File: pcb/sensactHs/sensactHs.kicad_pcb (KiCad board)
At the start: 2 copper layers, 100 x 86.5 mm, 185 parts, among them M1 Hole, M2 Hole, P1 CONN_01X08, P2 USB, P3 ESP01, P4 MicroSD, P5 SWD, P6 PWR+CANH, P7 CANH+CANL, P8 !24V!, SW1 PC5-Key, SW2 BOOT0, SW3 RESET, SW4 BOOT1, U1 ULN2803, U10 SRV05, U11 SRV05, U12 SRV05, U13 SRV05, U14 SRV05, U15 SRV05, U16 SRV05, U17 SRV05, U18 PCA9555, U19 PCA9555, U2 DRV8860woPad, U20 DRV8860woPad, U3 DRV8860woPad, U4 STM32F103RG, U5 LM2674, U6 SN65HVD230, U7 PCA9685, U8 DS2482, U9 PCA9685, X1 8MHz

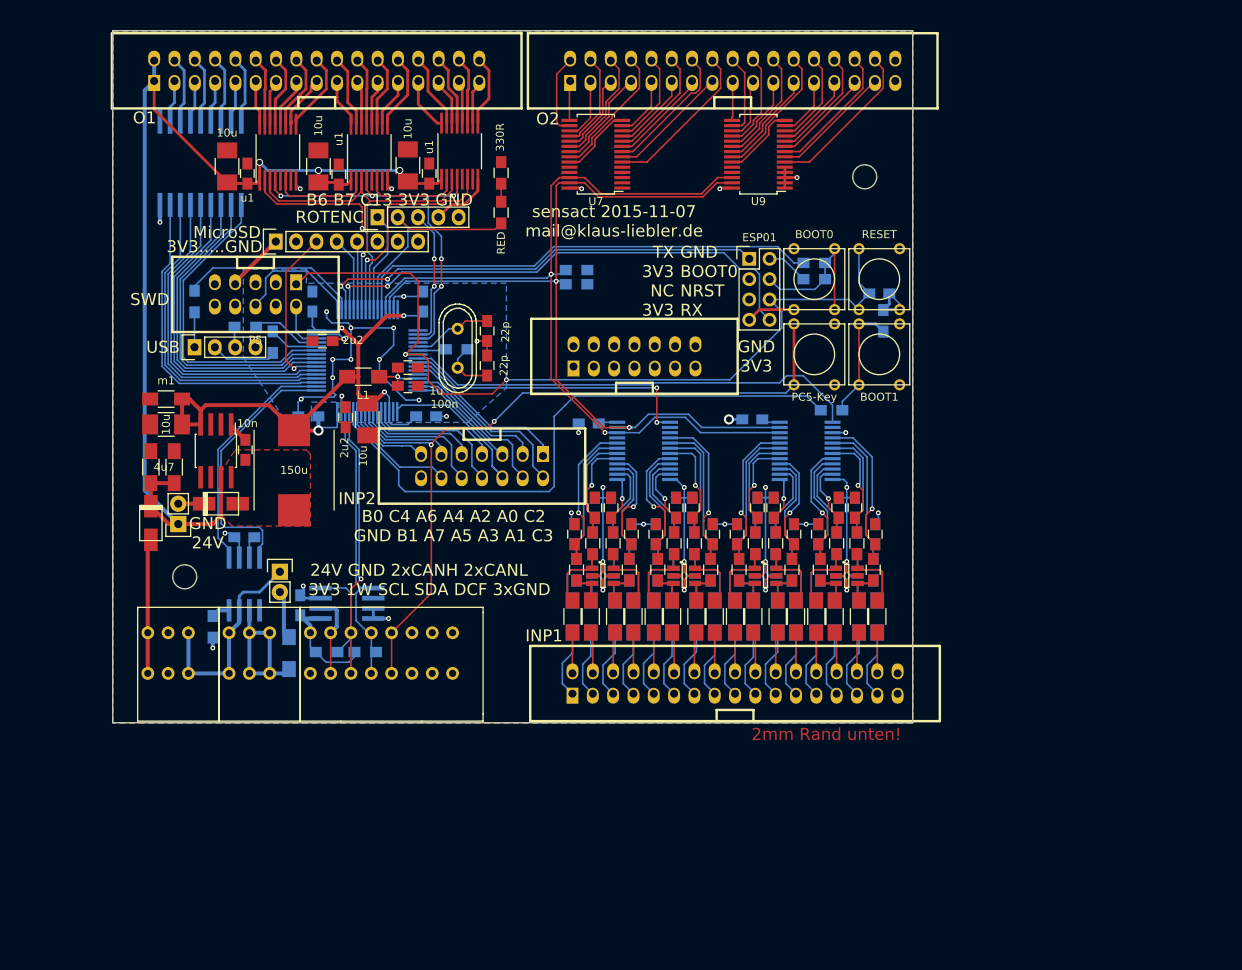
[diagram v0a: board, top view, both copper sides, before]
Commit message: new version of sensactHs
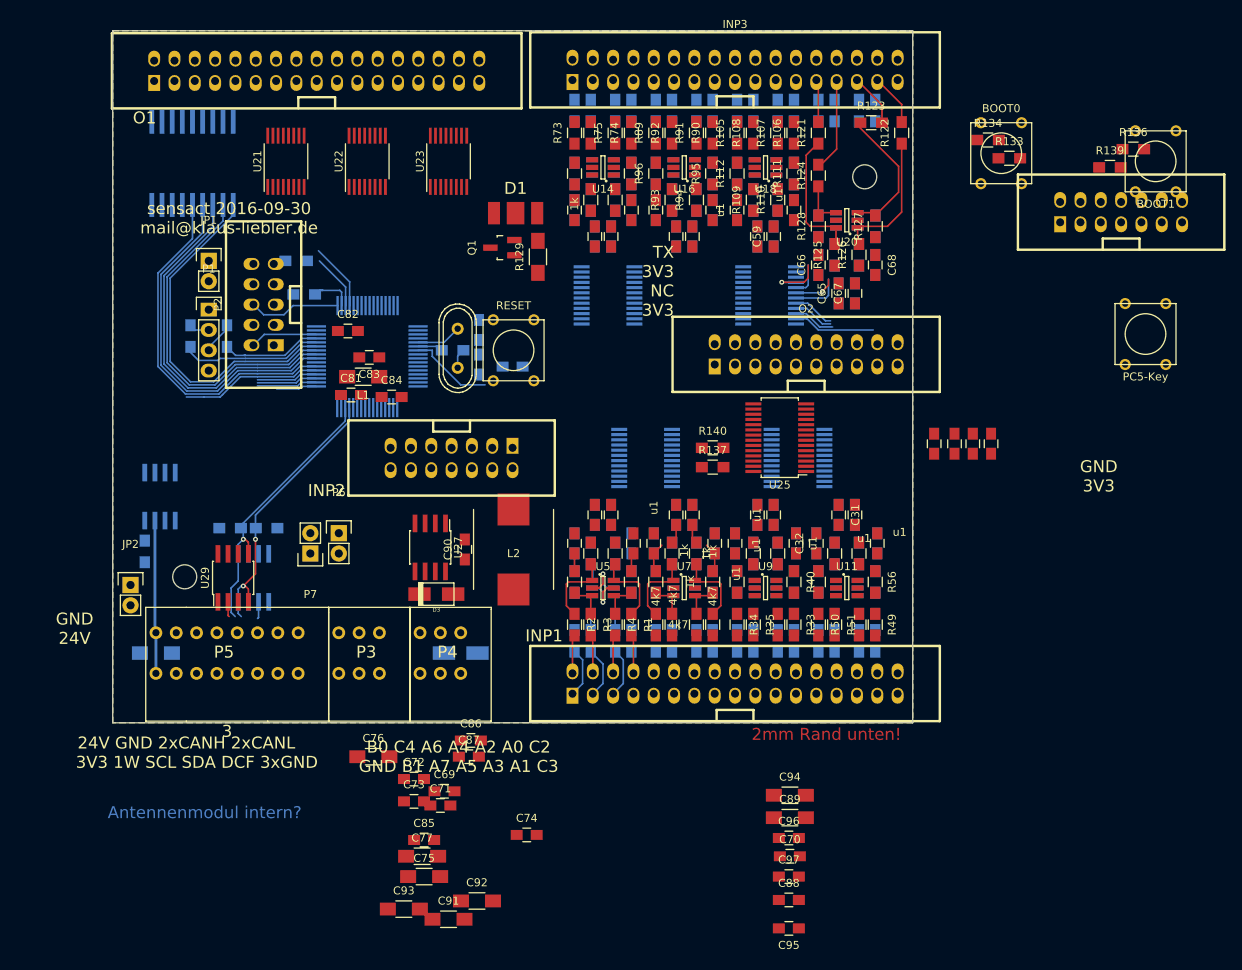
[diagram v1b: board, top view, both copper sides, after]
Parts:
- removed D16: RED, Resistors_SMD:R_0805_HandSoldering
- removed D17: SS14, kl_footprints:do214ac_handsolder
- removed D18: MBR0540, kl_footprints:do214ac_handsolder
- removed INP4: ROTENC, Pin_Headers:Pin_Header_Straight_1x05
- removed JP3: CAN_TERM, Pin_Headers:Pin_Header_Straight_1x02
- removed P8: !24V!, Pin_Headers:Pin_Header_Straight_1x02
- added C60: u1, Capacitors_SMD:C_0805_HandSoldering, F.Cu at (105.2, 41.9)
- added C61: u1, Capacitors_SMD:C_0805_HandSoldering, B.Cu at (112.8, 52.3)
- added C62: u1, Capacitors_SMD:C_0805_HandSoldering, B.Cu at (115.3, 48.8)
- added C63: u1, Capacitors_SMD:C_0805_HandSoldering, B.Cu at (110.7, 52.3)
- added C64: u1, Capacitors_SMD:C_0805_HandSoldering, B.Cu at (108.2, 48.8)
- added C65: u1, Capacitors_SMD:C_0805_HandSoldering, F.Cu at (110.7, 52.3)
- added C66: u1, Capacitors_SMD:C_0805_HandSoldering, F.Cu at (108.2, 48.8)
- added C67: u1, Capacitors_SMD:C_0805_HandSoldering, F.Cu at (112.8, 52.3)
- added C68: u1, Capacitors_SMD:C_0805_HandSoldering, F.Cu at (115.3, 48.8)
- added C69: u1, Capacitors_SMD:C_0805_HandSoldering, F.Cu at (61.5, 114.6)
- added C70: u1, Capacitors_SMD:C_0805_HandSoldering, F.Cu at (104.6, 122.7)
- added C71: u1, Capacitors_SMD:C_0805_HandSoldering, F.Cu at (61.0, 116.3)
- added C72: u1, Capacitors_SMD:C_0805_HandSoldering, F.Cu at (57.7, 113.0)
- added C73: u1, Capacitors_SMD:C_0805_HandSoldering, F.Cu at (57.7, 115.8)
- added C74: u1, Capacitors_SMD:C_0805_HandSoldering, F.Cu at (71.8, 120.0)
- added C75: 10u, Capacitors_SMD:C_1206_HandSoldering, F.Cu at (58.9, 125.2)
- added C76: 10u, Capacitors_SMD:C_1206_HandSoldering, F.Cu at (52.6, 110.2)
- added C77: 10u, Capacitors_SMD:C_1206_HandSoldering, F.Cu at (58.7, 122.7)
- added C78: 22p, Capacitors_SMD:C_0805_HandSoldering, B.Cu at (65.8, 56.9)
- added C79: 22p, Capacitors_SMD:C_0805_HandSoldering, B.Cu at (65.8, 61.2)
- added C80: u1, Capacitors_SMD:C_0805_HandSoldering, B.Cu at (70.0, 61.5)
- added C81: 2u2, Capacitors_SMD:C_0805_HandSoldering, F.Cu at (49.8, 65.0)
- added C82: 2u2, Capacitors_SMD:C_0805_HandSoldering, F.Cu at (49.4, 57.0)
- added C83: 1u, Capacitors_SMD:C_0805_HandSoldering, F.Cu at (52.1, 60.3)
- added C84: 1u, Capacitors_SMD:C_0805_HandSoldering, F.Cu at (54.9, 65.3)
- added C85: u1, Capacitors_SMD:C_0805_HandSoldering, F.Cu at (58.9, 120.7)
- added C86: u1, Capacitors_SMD:C_0805_HandSoldering, F.Cu at (64.8, 108.2)
- added C87: u1, Capacitors_SMD:C_0805_HandSoldering, F.Cu at (64.5, 110.2)
- added C88: u1, Capacitors_SMD:C_0805_HandSoldering, F.Cu at (104.5, 128.1)
- added C89: 10u, Capacitors_SMD:C_1206_HandSoldering, F.Cu at (104.6, 117.9)
- added C90: 10n, Capacitors_SMD:C_0805_HandSoldering, F.Cu at (64.0, 84.3)
- added C91: 4u7, Capacitors_SMD:C_1206_HandSoldering, F.Cu at (62.0, 130.6)
- added C92: 4u7, Capacitors_SMD:C_1206_HandSoldering, F.Cu at (65.5, 128.3)
- added C93: 10u, Capacitors_SMD:C_1206_HandSoldering, F.Cu at (56.4, 129.3)
- added C94: m1, Capacitors_SMD:C_1206_HandSoldering, F.Cu at (104.6, 115.1)
- added C95: 100n, Capacitors_SMD:C_0805_HandSoldering, F.Cu at (104.5, 131.7)
- added C96: u1, Capacitors_SMD:C_0805_HandSoldering, F.Cu at (104.5, 120.4)
- added C97: u1, Capacitors_SMD:C_0805_HandSoldering, F.Cu at (104.5, 125.2)
- added D1: RED, sensact:LED_5730, F.Cu at (70.4, 42.3)
- added D2: D, sensact:do214ac_handsolder, B.Cu at (63.5, 97.3)
- added D3: MBR0540, sensact:do214ac_handsolder, F.Cu at (60.5, 89.9)
- added INP3: PUSH_BUTTON_INPUT, w_conn_strip:vasch_strip_17x2, F.Cu at (97.8, 24.4)
- added JP1: JUMPER, Pin_Headers:Pin_Header_Straight_1x02, F.Cu at (32.0, 48.3)
- added JP2: CAN_TERM, Pin_Headers:Pin_Header_Straight_1x02, F.Cu at (22.2, 88.8)
- added Q1: Q_NPN_BEC, TO_SOT_Packages_SMD:SOT-23_Handsoldering, F.Cu at (68.7, 46.6)
- added R100: 4k7, Resistors_SMD:R_0805_HandSoldering, B.Cu at (103.1, 29.5)
- added R101: 1k, Resistors_SMD:R_0805_HandSoldering, B.Cu at (103.1, 40.6)
- added R102: 1k, Resistors_SMD:R_0805_HandSoldering, B.Cu at (100.1, 40.6)
- added R103: 1k, Resistors_SMD:R_0805_HandSoldering, B.Cu at (98.0, 37.3)
- added R104: 1k, Resistors_SMD:R_0805_HandSoldering, B.Cu at (105.2, 37.3)
- added R105: 4k7, Resistors_SMD:R_0805_HandSoldering, F.Cu at (98.0, 32.3)
- added R106: 4k7, Resistors_SMD:R_0805_HandSoldering, F.Cu at (105.2, 32.3)
- added R107: 4k7, Resistors_SMD:R_0805_HandSoldering, F.Cu at (103.1, 32.3)
- added R108: 4k7, Resistors_SMD:R_0805_HandSoldering, F.Cu at (100.1, 32.3)
- added R109: 1k, Resistors_SMD:R_0805_HandSoldering, F.Cu at (100.1, 40.6)
- added R110: 1k, Resistors_SMD:R_0805_HandSoldering, F.Cu at (103.1, 40.6)
- added R111: 1k, Resistors_SMD:R_0805_HandSoldering, F.Cu at (105.2, 37.3)
- added R112: 1k, Resistors_SMD:R_0805_HandSoldering, F.Cu at (98.0, 37.3)
- added R113: 4k7, Resistors_SMD:R_0805_HandSoldering, B.Cu at (115.3, 29.5)
- added R114: 4k7, Resistors_SMD:R_0805_HandSoldering, B.Cu at (108.2, 29.5)
- added R115: 4k7, Resistors_SMD:R_0805_HandSoldering, B.Cu at (110.2, 29.5)
- added R116: 4k7, Resistors_SMD:R_0805_HandSoldering, B.Cu at (113.3, 29.5)
- added R117: 1k, Resistors_SMD:R_0805_HandSoldering, B.Cu at (113.3, 47.5)
- added R118: 1k, Resistors_SMD:R_0805_HandSoldering, B.Cu at (110.2, 47.5)
- added R119: 1k, Resistors_SMD:R_0805_HandSoldering, B.Cu at (108.2, 43.9)
- added R120: 1k, Resistors_SMD:R_0805_HandSoldering, B.Cu at (115.3, 43.9)
- added R121: 4k7, Resistors_SMD:R_0805_HandSoldering, F.Cu at (108.2, 32.3)
- added R122: 4k7, Resistors_SMD:R_0805_HandSoldering, F.Cu at (118.6, 32.3)
- added R123: 4k7, Resistors_SMD:R_0805_HandSoldering, F.Cu at (114.8, 31.0)
- added R124: 4k7, Resistors_SMD:R_0805_HandSoldering, F.Cu at (108.2, 37.6)
- added R125: 1k, Resistors_SMD:R_0805_HandSoldering, F.Cu at (110.2, 47.5)
- added R126: 1k, Resistors_SMD:R_0805_HandSoldering, F.Cu at (113.3, 47.5)
- added R127: 1k, Resistors_SMD:R_0805_HandSoldering, F.Cu at (115.3, 43.9)
- added R128: 1k, Resistors_SMD:R_0805_HandSoldering, F.Cu at (108.2, 43.9)
- added R129: 330R, Resistors_SMD:R_1206_HandSoldering, F.Cu at (73.2, 47.8)
- added R130: 1k, Resistors_SMD:R_0805_HandSoldering, B.Cu at (43.9, 52.5)
- added R131: 22R, Resistors_SMD:R_0805_HandSoldering, B.Cu at (29.7, 57.7)
- added R132: 22R, Resistors_SMD:R_0805_HandSoldering, B.Cu at (34.3, 57.7)
- added R133: 10k, Resistors_SMD:R_0805_HandSoldering, F.Cu at (132.1, 35.4)
- added R134: 10k, Resistors_SMD:R_0805_HandSoldering, F.Cu at (129.4, 33.1)
- added R135: 220R, Resistors_SMD:R_0805_HandSoldering, B.Cu at (62.5, 59.4)
- added R136: 10k, Resistors_SMD:R_0805_HandSoldering, F.Cu at (147.6, 34.3)
- added R137: 4k7, Resistors_SMD:R_0805_HandSoldering, F.Cu at (95.0, 74.0)
- added R138: 4k7, Resistors_SMD:R_0805_HandSoldering, B.Cu at (39.2, 81.7)
- added R139: 10k, Resistors_SMD:R_0805_HandSoldering, F.Cu at (144.7, 36.6)
- added R140: 4k7, Resistors_SMD:R_0805_HandSoldering, F.Cu at (95.0, 71.6)
- added R141: 4k7, Resistors_SMD:R_0805_HandSoldering, B.Cu at (34.7, 81.7)
- added R142: 10k, Resistors_SMD:R_0805_HandSoldering, B.Cu at (24.0, 84.6)
- added R143: 120R, Resistors_SMD:R_1206_HandSoldering, B.Cu at (25.4, 97.3)
- added R144: 1k, Resistors_SMD:R_0805_HandSoldering, B.Cu at (42.9, 48.3)
- added R28: 4k7, Resistors_SMD:R_0805_HandSoldering, B.Cu at (89.9, 95.8)
- added R29: 1k, Resistors_SMD:R_0805_HandSoldering, B.Cu at (89.9, 84.8)
- added R82: 4k7, Resistors_SMD:R_0805_HandSoldering, B.Cu at (87.9, 29.5)
- added R83: 4k7, Resistors_SMD:R_0805_HandSoldering, B.Cu at (89.9, 29.5)
- added R84: 4k7, Resistors_SMD:R_0805_HandSoldering, B.Cu at (93.0, 29.5)
- added R85: 1k, Resistors_SMD:R_0805_HandSoldering, B.Cu at (93.0, 40.6)
- added R86: 1k, Resistors_SMD:R_0805_HandSoldering, B.Cu at (89.9, 40.6)
- added R87: 1k, Resistors_SMD:R_0805_HandSoldering, B.Cu at (87.9, 37.3)
- added R88: 1k, Resistors_SMD:R_0805_HandSoldering, B.Cu at (95.0, 37.3)
- added R89: 4k7, Resistors_SMD:R_0805_HandSoldering, F.Cu at (87.9, 32.3)
- added R90: 4k7, Resistors_SMD:R_0805_HandSoldering, F.Cu at (95.0, 32.3)
- added R91: 4k7, Resistors_SMD:R_0805_HandSoldering, F.Cu at (93.0, 32.3)
- added R92: 4k7, Resistors_SMD:R_0805_HandSoldering, F.Cu at (89.9, 32.3)
- added R93: 1k, Resistors_SMD:R_0805_HandSoldering, F.Cu at (89.9, 40.6)
- added R94: 1k, Resistors_SMD:R_0805_HandSoldering, F.Cu at (93.0, 40.6)
- added R95: 1k, Resistors_SMD:R_0805_HandSoldering, F.Cu at (95.0, 37.3)
- added R96: 1k, Resistors_SMD:R_0805_HandSoldering, F.Cu at (87.9, 37.3)
- added R97: 4k7, Resistors_SMD:R_0805_HandSoldering, B.Cu at (105.2, 29.5)
- added R98: 4k7, Resistors_SMD:R_0805_HandSoldering, B.Cu at (98.0, 29.5)
- added R99: 4k7, Resistors_SMD:R_0805_HandSoldering, B.Cu at (100.1, 29.5)
- added U21: DRV8860woPad, sensact:TSSOP-16_4.4x5mm_Pitch0.65mm_handsolder, F.Cu at (41.7, 35.8)
- added U22: DRV8860woPad, sensact:TSSOP-16_4.4x5mm_Pitch0.65mm_handsolder, F.Cu at (51.8, 35.8)
- added U23: DRV8860woPad, sensact:TSSOP-16_4.4x5mm_Pitch0.65mm_handsolder, F.Cu at (62.0, 35.8)
- added U24: ULN2803, sensact:SOIC-18_7.5x11.6mm_Pitch1.27mm_handsolder, B.Cu at (30.0, 36.1)
- added U25: PCA9685, sensact:TSSOP-28_4.4x9.7mm_Pitch0.65mm_handsolder, F.Cu at (103.4, 70.4)
- added U26: STM32F103RG, sensact:LQFP-64_10x10mm_Pitch0.5mm_handsolder, B.Cu at (51.8, 60.2)
- added U27: LM2674, sensact:SOIC-8_3.9x4.9mm_Pitch1.27mm_handsolder, F.Cu at (59.7, 84.1)
- added U28: SN65HVD230, sensact:SOIC-8_3.9x4.9mm_Pitch1.27mm_handsolder, B.Cu at (25.9, 77.7)
- added U29: DS2482, sensact:SOIC-8_3.9x4.9mm_Pitch1.27mm_handsolder, F.Cu at (35.1, 87.9)
- added U30: DS2482, sensact:SOIC-8_3.9x4.9mm_Pitch1.27mm_handsolder, B.Cu at (37.6, 87.9)
- C10, C11, C12, C17, C40, C45, C53, C9, R69, R70, R71: moved to B.Cu
- C13, C14, C15, C41, C49, C5, C57, C58, C6, C7, C8, R77, R78, R79: moved to F.Cu
- C18, C19, C36: value 10u -> u1; footprint Capacitors_SMD:C_1210_HandSoldering -> Capacitors_SMD:C_0805_HandSoldering; moved to B.Cu
- C20: value 22p -> u1; moved to B.Cu
- C21: value 22p -> u1
- C22, C29, C30: value 100n -> u1; moved to F.Cu
- C23, C24: value 2u2 -> u1
- C25: value 100n -> u1; moved to B.Cu
- C26: value 1u -> u1; moved to B.Cu
- C27, C28, C38: value 100n -> u1
- C31, C59: value 10u -> u1; footprint Capacitors_SMD:C_1210_HandSoldering -> Capacitors_SMD:C_0805_HandSoldering
- C32: value 4u7 -> u1; footprint Capacitors_SMD:C_1206_HandSoldering -> Capacitors_SMD:C_0805_HandSoldering
- C33: value 4u7 -> u1; footprint Capacitors_SMD:C_1206_HandSoldering -> Capacitors_SMD:C_0805_HandSoldering; moved to B.Cu
- C34: value 10n -> u1; moved to B.Cu
- C37: value m1 -> u1; footprint Capacitors_SMD:C_1206_HandSoldering -> Capacitors_SMD:C_0805_HandSoldering; moved to B.Cu
- L2: footprint kl_footprints:Inductor_CD104_handsolder -> sensact:Inductor_CD104_handsolder
- O2: value PWM OUTPUTS -> PWM_OUTPUTS; footprint w_conn_strip:vasch_strip_17x2 -> w_conn_strip:vasch_strip_10x2
- P1: value CONN_01X08 -> USB; footprint kl_footprints:KF141R-8p -> Pin_Headers:Pin_Header_Straight_1x04
- P2: value USB -> SWD; footprint Pin_Headers:Pin_Header_Straight_1x04 -> w_conn_strip:vasch_strip_5x2
- P3: value ESP01 -> 2; footprint Pin_Headers:Pin_Header_Straight_2x04 -> sensact:KF141R-3p
- P4: value MicroSD -> 1; footprint Pin_Headers:Pin_Header_Straight_1x08 -> sensact:KF141R-3p
- P5: value SWD -> 3; footprint w_conn_strip:vasch_strip_5x2 -> sensact:KF141R-8p
- P6: value PWR+CANH -> !24V!; footprint kl_footprints:KF141R-3p -> Pin_Headers:Pin_Header_Straight_1x02
- P7: value CANH+CANL -> 5V_IN; footprint kl_footprints:KF141R-3p -> Pin_Headers:Pin_Header_Straight_1x02
- R1, R10, R11, R12, R2, R3, R33, R34, R35, R4, R41, R42, R43, R49, R50, R51, R57, R58, R59, R9: footprint Resistors_SMD:R_1206_HandSoldering -> Resistors_SMD:R_0805_HandSoldering
- R16: value 330R -> 1k; moved to B.Cu
- R17, R18: value 22R -> 4k7; moved to F.Cu
- R19, R20: value 10k -> 4k7; moved to F.Cu
- R21: value 220R -> 1k; moved to F.Cu
- R22, R23, R80: value 4k7 -> 1k; moved to F.Cu
- R24: value 10k -> 1k; moved to F.Cu
- R25, R26: value 10k -> 4k7
- R27: value 120R -> 4k7; footprint Resistors_SMD:R_1206_HandSoldering -> Resistors_SMD:R_0805_HandSoldering
- R32, R48, R64: value 4k7 -> 1k; footprint Resistors_SMD:R_1206_HandSoldering -> Resistors_SMD:R_0805_HandSoldering; moved to B.Cu
- R36, R44, R52, R60: value 1k -> 4k7
- R40, R56: value 4k7 -> 1k; footprint Resistors_SMD:R_1206_HandSoldering -> Resistors_SMD:R_0805_HandSoldering; moved to F.Cu
- R65, R66, R67: footprint Resistors_SMD:R_1206_HandSoldering -> Resistors_SMD:R_0805_HandSoldering; moved to B.Cu
- R68: value 1k -> 4k7; moved to B.Cu
- R72: value 4k7 -> 1k; footprint Resistors_SMD:R_1206_HandSoldering -> Resistors_SMD:R_0805_HandSoldering
- R73, R74, R75: footprint Resistors_SMD:R_1206_HandSoldering -> Resistors_SMD:R_0805_HandSoldering; moved to F.Cu
- R76: value 1k -> 4k7; moved to F.Cu
- U1: value ULN2803 -> PCA9555; footprint kl_footprints:SOIC-18_7.5x11.6mm_Pitch1.27mm_handsolder -> sensact:TSSOP-24_4.4x7.8mm_Pitch0.65mm_handsolder
- U10, U12: footprint kl_footprints:SOT-23-6_handsolder -> sensact:SOT-23-6_handsolder; moved to B.Cu
- U11: footprint kl_footprints:SOT-23-6_handsolder -> sensact:SOT-23-6_handsolder; moved to F.Cu
- U13, U14, U15, U16, U17: footprint kl_footprints:SOT-23-6_handsolder -> sensact:SOT-23-6_handsolder
- U18: value PCA9555 -> SRV05; footprint kl_footprints:TSSOP-24_4.4x7.8mm_Pitch0.65mm_handsolder -> sensact:SOT-23-6_handsolder; moved to F.Cu
- U19: value PCA9555 -> SRV05; footprint kl_footprints:TSSOP-24_4.4x7.8mm_Pitch0.65mm_handsolder -> sensact:SOT-23-6_handsolder
- U2, U3: value DRV8860woPad -> PCA9555; footprint kl_footprints:TSSOP-16_4.4x5mm_Pitch0.65mm_handsolder -> sensact:TSSOP-24_4.4x7.8mm_Pitch0.65mm_handsolder; moved to B.Cu
- U20: value DRV8860woPad -> SRV05; footprint kl_footprints:TSSOP-16_4.4x5mm_Pitch0.65mm_handsolder -> sensact:SOT-23-6_handsolder
- U4: value STM32F103RG -> PCA9555; footprint kl_footprints:LQFP-64_10x10mm_Pitch0.5mm_handsolder -> sensact:TSSOP-24_4.4x7.8mm_Pitch0.65mm_handsolder
- U5: value LM2674 -> SRV05; footprint kl_footprints:SOIC-8_3.9x4.9mm_Pitch1.27mm_handsolder -> sensact:SOT-23-6_handsolder
- U6: value SN65HVD230 -> SRV05; footprint kl_footprints:SOIC-8_3.9x4.9mm_Pitch1.27mm_handsolder -> sensact:SOT-23-6_handsolder
- U7, U9: value PCA9685 -> SRV05; footprint kl_footprints:TSSOP-28_4.4x9.7mm_Pitch0.65mm_handsolder -> sensact:SOT-23-6_handsolder
- U8: value DS2482 -> SRV05; footprint kl_footprints:SOIC-8_3.9x4.9mm_Pitch1.27mm_handsolder -> sensact:SOT-23-6_handsolder
- moved C36 90.1 mm to (115.6, 83.6), turned to 90 degrees
- moved C32 83.7 mm to (108.0, 83.6)
- moved C33 83.3 mm to (110.7, 80.0), turned to 270 degrees
- moved U2 75.4 mm to (105.7, 72.9), turned to 180 degrees
- moved C29 72.9 mm to (112.8, 80.0), turned to 270 degrees
- moved C19 72.7 mm to (92.5, 80.0), turned to 270 degrees
- moved C34 72.3 mm to (108.0, 83.6)
- moved R67 71.6 mm to (79.8, 29.5), turned to 90 degrees
- moved R73 71.3 mm to (77.7, 32.3), turned to 90 degrees
- moved R66 71.1 mm to (77.7, 29.5), turned to 90 degrees
- moved C35 70.3 mm to (112.8, 80.0), turned to 270 degrees
- moved R30 70.2 mm to (93.0, 84.8), turned to 270 degrees
- moved C17 68.5 mm to (90.4, 80.0), turned to 270 degrees
- moved P3 68.4 mm to (52.1, 97.3)
- moved R65 67.3 mm to (84.8, 29.5), turned to 90 degrees
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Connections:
- C1 pad 1: GND -> +3V3
- C1 pad 2: /01 input/ESDProtection1/O1 -> GND
- C10 pad 1: /01 input/ESDProtection3/O4 -> /01 input/ESDProtection2/O4
- C11 pad 2: /01 input/ESDProtection3/O2 -> /01 input/ESDProtection2/O2
- C12 pad 1: /01 input/ESDProtection3/O3 -> /01 input/ESDProtection2/O3
- C13 pad 2: /01 input/ESDProtection4/O1 -> /01 input/ESDProtection3/O1
- C14 pad 1: /01 input/ESDProtection4/O4 -> /01 input/ESDProtection3/O4
- C15 pad 2: /01 input/ESDProtection4/O2 -> /01 input/ESDProtection3/O2
- C16 pad 1: VCC -> /01 input/ESDProtection3/O3
- C17 pad 1: VCC -> GND
- C17 pad 2: GND -> /01 input/ESDProtection4/O1
- C18 pad 1: VCC -> /01 input/ESDProtection4/O4
- C19 pad 1: VCC -> GND
- C19 pad 2: GND -> /01 input/ESDProtection4/O2
- C2 pad 1: /01 input/ESDProtection1/O4 -> +3V3
- C20 pad 1: Net-(C20-Pad1) -> /01 input/ESDProtection4/O3
- C21 pad 1: Net-(C21-Pad1) -> GND
- C21 pad 2: GND -> /01 input/ESDProtection5/O1
- C22 pad 1: /03 cpu/NRST -> /01 input/ESDProtection5/O4
- C23 pad 1: Net-(C23-Pad1) -> GND
- C23 pad 2: GND -> /01 input/ESDProtection5/O2
- C24 pad 1: Net-(C24-Pad1) -> /01 input/ESDProtection5/O3
- C25 pad 1: Net-(C25-Pad1) -> GND
- C25 pad 2: GND -> /01 input/ESDProtection6/O1
- C26 pad 1: Net-(C25-Pad1) -> /01 input/ESDProtection6/O4
- C27 pad 1: +3V3 -> GND
- C27 pad 2: GND -> /01 input/ESDProtection6/O2
- C28 pad 1: +3V3 -> /01 input/ESDProtection6/O3
- C29 pad 1: +3V3 -> GND
- C29 pad 2: GND -> /01 input/ESDProtection7/O1
- C3 pad 1: GND -> +3V3
- C3 pad 2: /01 input/ESDProtection1/O2 -> GND
- C30 pad 1: +3V3 -> /01 input/ESDProtection7/O4
- C31 pad 1: +3V3 -> GND
- C31 pad 2: GND -> /01 input/ESDProtection7/O2
- C32 pad 1: VCC -> /01 input/ESDProtection7/O3
- C33 pad 1: VCC -> GND
- C33 pad 2: GND -> /01 input/ESDProtection8/O1
- C34 pad 1: /04 power/V_SW -> /01 input/ESDProtection8/O4
- C34 pad 2: /04 power/V_CB -> GND
- C35 pad 1: +3V3 -> GND
- C35 pad 2: GND -> /01 input/ESDProtection8/O2
- C36 pad 1: +3V3 -> /01 input/ESDProtection8/O3
- C37 pad 1: +3V3 -> GND
- C37 pad 2: GND -> /01 input/ESDProtection9/O1
- C38 pad 1: +3V3 -> /01 input/ESDProtection9/O4
- C39 pad 1: +3V3 -> GND
- C39 pad 2: GND -> /01 input/ESDProtection9/O2
- C4 pad 1: /01 input/ESDProtection1/O3 -> +3V3
- C40 pad 1: VCC -> /01 input/ESDProtection9/O3
- C41 pad 1: /01 input/ESDProtection4/O3 -> GND
- C41 pad 2: GND -> /01 input/ESDProtection10/O1
- C42 pad 1: GND -> /01 input/ESDProtection10/O4
- C42 pad 2: /01 input/ESDProtection5/O1 -> GND
- C43 pad 1: /01 input/ESDProtection5/O4 -> GND
- C43 pad 2: GND -> /01 input/ESDProtection10/O2
- C44 pad 1: GND -> /01 input/ESDProtection10/O3
- C44 pad 2: /01 input/ESDProtection5/O2 -> GND
- C45 pad 1: /01 input/ESDProtection5/O3 -> GND
- C45 pad 2: GND -> /01 input/ESDProtection11/O1
- C46 pad 1: GND -> /01 input/ESDProtection11/O4
- C46 pad 2: /01 input/ESDProtection6/O1 -> GND
- C47 pad 1: /01 input/ESDProtection6/O4 -> GND
- C47 pad 2: GND -> /01 input/ESDProtection11/O2
- C48 pad 1: GND -> /01 input/ESDProtection11/O3
- C48 pad 2: /01 input/ESDProtection6/O2 -> GND
- C49 pad 1: /01 input/ESDProtection6/O3 -> GND
- C49 pad 2: GND -> /01 input/ESDProtection12/O1
- C5 pad 2: /01 input/ESDProtection2/O1 -> /01 input/ESDProtection1/O1
- C50 pad 1: GND -> /01 input/ESDProtection12/O4
- C50 pad 2: /01 input/ESDProtection7/O1 -> GND
- C51 pad 1: /01 input/ESDProtection7/O4 -> GND
- C51 pad 2: GND -> /01 input/ESDProtection12/O2
- C52 pad 1: GND -> /01 input/ESDProtection12/O3
- C52 pad 2: /01 input/ESDProtection7/O2 -> GND
- C53 pad 1: /01 input/ESDProtection7/O3 -> GND
- C53 pad 2: GND -> /01 input/ESDProtection13/O1
- C54 pad 1: GND -> /01 input/ESDProtection13/O4
- C54 pad 2: /01 input/ESDProtection8/O1 -> GND
- C55 pad 1: /01 input/ESDProtection8/O4 -> GND
- C55 pad 2: GND -> /01 input/ESDProtection13/O2
- C56 pad 1: GND -> /01 input/ESDProtection13/O3
- C56 pad 2: /01 input/ESDProtection8/O2 -> GND
- C57 pad 1: /01 input/ESDProtection8/O3 -> GND
- C57 pad 2: GND -> /01 input/ESDProtection14/O1
- C58 pad 1: +3V3 -> /01 input/ESDProtection14/O4
- C59 pad 1: VCC -> GND
- C59 pad 2: GND -> /01 input/ESDProtection14/O2
- C6 pad 1: /01 input/ESDProtection2/O4 -> /01 input/ESDProtection1/O4
- C7 pad 2: /01 input/ESDProtection2/O2 -> /01 input/ESDProtection1/O2
- C8 pad 1: /01 input/ESDProtection2/O3 -> /01 input/ESDProtection1/O3
- C9 pad 2: /01 input/ESDProtection3/O1 -> /01 input/ESDProtection2/O1
- L1 pad 1: Net-(C25-Pad1) -> Net-(C83-Pad1)
- O1 pad 10: /02 output/O1.8 -> Net-(O1-Pad10)
- O1 pad 3: /02 output/O1.1 -> Net-(O1-Pad3)
- O1 pad 4: /02 output/O1.2 -> Net-(O1-Pad4)
- O1 pad 5: /02 output/O1.3 -> Net-(O1-Pad5)
- O1 pad 6: /02 output/O1.4 -> Net-(O1-Pad6)
- O1 pad 7: /02 output/O1.5 -> Net-(O1-Pad7)
- O1 pad 8: /02 output/O1.6 -> Net-(O1-Pad8)
- O1 pad 9: /02 output/O1.7 -> Net-(O1-Pad9)
- O2 pad 16: Net-(O2-Pad16) -> GND
- O2 pad 17: Net-(O2-Pad17) -> GND
- O2 pad 18: Net-(O2-Pad18) -> GND
- O2 pad 19: Net-(O2-Pad19) -> GND
- O2 pad 20: Net-(O2-Pad20) -> GND
- P1 pad 1: +3V3 -> Net-(P1-Pad1)
- P1 pad 2: /03 cpu/1W -> Net-(P1-Pad2)
- P1 pad 3: SCL2 -> Net-(P1-Pad3)
- P1 pad 4: SDA2 -> GND
- P2 pad 1: Net-(P2-Pad1) -> /03 cpu/NRST
- P2 pad 2: Net-(P2-Pad2) -> /03 cpu/SWDIO
- P2 pad 3: Net-(P2-Pad3) -> GND
- P3 pad 1: /03 cpu/PC10 -> /04 power/CANH
- P3 pad 2: GND -> /04 power/CANH
- P3 pad 3: +3V3 -> /04 power/CANL
- P4 pad 1: +3V3 -> /04 power/CANL
- P4 pad 2: (no net) -> GND
- P4 pad 3: /03 cpu/PC8 -> +5V
- P5 pad 1: /03 cpu/NRST -> +3V3
- P5 pad 2: /03 cpu/SWDIO -> /04 power/1Wa
- P5 pad 3: GND -> SCL2
- P5 pad 4: GND -> SDA2
- P5 pad 5: (no net) -> /04 power/DCF77
- P5 pad 6: /03 cpu/SWCLK -> /04 power/1Wb
- P5 pad 7: +3V3 -> VCC
- P5 pad 8: +3V3 -> GND
- P7 pad 1: /04 power/CANH -> +5V
- P7 pad 2: /04 power/CANL -> GND
- R16 pad 1: GND -> /01 input/ESDProtection2/O4
- R16 pad 2: Net-(D16-Pad1) -> Net-(R12-Pad1)
- R17 pad 1: Net-(P2-Pad2) -> Net-(R17-Pad1)
- R17 pad 2: /03 cpu/PA11 -> /01 input/ESDProtection3/I1
- R18 pad 1: Net-(P2-Pad3) -> Net-(R18-Pad1)
- R18 pad 2: /03 cpu/PA12 -> /01 input/ESDProtection3/I2
- R19 pad 1: /03 cpu/BOOT0 -> Net-(R19-Pad1)
- R19 pad 2: GND -> /01 input/ESDProtection3/I3
- R20 pad 2: /03 cpu/BOOT0 -> /01 input/ESDProtection3/I4
- R21 pad 1: Net-(R21-Pad1) -> /01 input/ESDProtection3/O1
- R21 pad 2: Net-(C21-Pad1) -> Net-(R17-Pad1)
- R22 pad 1: +3V3 -> /01 input/ESDProtection3/O2
- R22 pad 2: SCL2 -> Net-(R18-Pad1)
- R23 pad 1: +3V3 -> /01 input/ESDProtection3/O3
- R23 pad 2: SDA2 -> Net-(R19-Pad1)
- R24 pad 1: Net-(R24-Pad1) -> /01 input/ESDProtection3/O4
- R24 pad 2: /03 cpu/PB2 -> Net-(R20-Pad1)
- R25 pad 1: GND -> Net-(R25-Pad1)
- R25 pad 2: Net-(R24-Pad1) -> /01 input/ESDProtection4/I1
- R26 pad 2: GND -> /01 input/ESDProtection4/I2
- R27 pad 1: Net-(JP3-Pad2) -> Net-(R27-Pad1)
- R27 pad 2: /04 power/CANL -> /01 input/ESDProtection4/I3
- R30 pad 1: Net-(P2-Pad1) -> /01 input/ESDProtection4/O2
- R30 pad 2: /03 cpu/PA15 -> Net-(R26-Pad1)
- R31 pad 1: /01 input/ESDProtection2/O4 -> /01 input/ESDProtection4/O3
- R31 pad 2: Net-(R12-Pad1) -> Net-(R27-Pad1)
- R32 pad 1: Net-(R32-Pad1) -> /01 input/ESDProtection4/O4
- R32 pad 2: /01 input/ESDProtection3/I1 -> Net-(R28-Pad1)
- R33 pad 2: /01 input/ESDProtection3/I2 -> /01 input/ESDProtection5/I1
- R34 pad 2: /01 input/ESDProtection3/I3 -> /01 input/ESDProtection5/I2
- R35 pad 2: /01 input/ESDProtection3/I4 -> /01 input/ESDProtection5/I3
- R36 pad 1: /01 input/ESDProtection3/O1 -> Net-(R36-Pad1)
- R36 pad 2: Net-(R32-Pad1) -> /01 input/ESDProtection5/I4
- R37 pad 1: /01 input/ESDProtection3/O2 -> /01 input/ESDProtection5/O1
- R38 pad 1: /01 input/ESDProtection3/O3 -> /01 input/ESDProtection5/O2
- R39 pad 1: /01 input/ESDProtection3/O4 -> /01 input/ESDProtection5/O3
- R40 pad 1: Net-(R40-Pad1) -> /01 input/ESDProtection5/O4
- R40 pad 2: /01 input/ESDProtection4/I1 -> Net-(R36-Pad1)
- R41 pad 2: /01 input/ESDProtection4/I2 -> /01 input/ESDProtection6/I1
- R42 pad 2: /01 input/ESDProtection4/I3 -> /01 input/ESDProtection6/I2
- R43 pad 2: /01 input/ESDProtection4/I4 -> /01 input/ESDProtection6/I3
- R44 pad 1: /01 input/ESDProtection4/O1 -> Net-(R44-Pad1)
- R44 pad 2: Net-(R40-Pad1) -> /01 input/ESDProtection6/I4
- R45 pad 1: /01 input/ESDProtection4/O2 -> /01 input/ESDProtection6/O1
- R46 pad 1: /01 input/ESDProtection4/O3 -> /01 input/ESDProtection6/O2
- R47 pad 1: /01 input/ESDProtection4/O4 -> /01 input/ESDProtection6/O3
- R48 pad 1: Net-(R48-Pad1) -> /01 input/ESDProtection6/O4
- R48 pad 2: /01 input/ESDProtection5/I1 -> Net-(R44-Pad1)
- R49 pad 2: /01 input/ESDProtection5/I2 -> /01 input/ESDProtection7/I1
- R50 pad 2: /01 input/ESDProtection5/I3 -> /01 input/ESDProtection7/I2
- R51 pad 2: /01 input/ESDProtection5/I4 -> /01 input/ESDProtection7/I3
- R52 pad 1: /01 input/ESDProtection5/O1 -> Net-(R52-Pad1)
- R52 pad 2: Net-(R48-Pad1) -> /01 input/ESDProtection7/I4
- R53 pad 1: /01 input/ESDProtection5/O2 -> /01 input/ESDProtection7/O1
- R54 pad 1: /01 input/ESDProtection5/O3 -> /01 input/ESDProtection7/O2
- R55 pad 1: /01 input/ESDProtection5/O4 -> /01 input/ESDProtection7/O3
- R56 pad 1: Net-(R56-Pad1) -> /01 input/ESDProtection7/O4
- R56 pad 2: /01 input/ESDProtection6/I1 -> Net-(R52-Pad1)
- R57 pad 2: /01 input/ESDProtection6/I2 -> /01 input/ESDProtection8/I1
- R58 pad 2: /01 input/ESDProtection6/I3 -> /01 input/ESDProtection8/I2
- R59 pad 2: /01 input/ESDProtection6/I4 -> /01 input/ESDProtection8/I3
- R60 pad 1: /01 input/ESDProtection6/O1 -> Net-(R60-Pad1)
- R60 pad 2: Net-(R56-Pad1) -> /01 input/ESDProtection8/I4
- R61 pad 1: /01 input/ESDProtection6/O2 -> /01 input/ESDProtection8/O1
- R62 pad 1: /01 input/ESDProtection6/O3 -> /01 input/ESDProtection8/O2
- R63 pad 1: /01 input/ESDProtection6/O4 -> /01 input/ESDProtection8/O3
- R64 pad 1: Net-(R64-Pad1) -> /01 input/ESDProtection8/O4
- R64 pad 2: /01 input/ESDProtection7/I1 -> Net-(R60-Pad1)
- R65 pad 2: /01 input/ESDProtection7/I2 -> /01 input/ESDProtection9/I1
- R66 pad 2: /01 input/ESDProtection7/I3 -> /01 input/ESDProtection9/I2
- R67 pad 2: /01 input/ESDProtection7/I4 -> /01 input/ESDProtection9/I3
- R68 pad 1: /01 input/ESDProtection7/O1 -> Net-(R68-Pad1)
- R68 pad 2: Net-(R64-Pad1) -> /01 input/ESDProtection9/I4
- R69 pad 1: /01 input/ESDProtection7/O2 -> /01 input/ESDProtection9/O1
- R70 pad 1: /01 input/ESDProtection7/O3 -> /01 input/ESDProtection9/O2
- R71 pad 1: /01 input/ESDProtection7/O4 -> /01 input/ESDProtection9/O3
- R72 pad 1: Net-(R72-Pad1) -> /01 input/ESDProtection9/O4
- R72 pad 2: /01 input/ESDProtection8/I1 -> Net-(R68-Pad1)
- R73 pad 2: /01 input/ESDProtection8/I2 -> /01 input/ESDProtection10/I1
- R74 pad 2: /01 input/ESDProtection8/I3 -> /01 input/ESDProtection10/I2
- R75 pad 2: /01 input/ESDProtection8/I4 -> /01 input/ESDProtection10/I3
- R76 pad 1: /01 input/ESDProtection8/O1 -> Net-(R76-Pad1)
- R76 pad 2: Net-(R72-Pad1) -> /01 input/ESDProtection10/I4
- R77 pad 1: /01 input/ESDProtection8/O2 -> /01 input/ESDProtection10/O1
- R78 pad 1: /01 input/ESDProtection8/O3 -> /01 input/ESDProtection10/O2
- R79 pad 1: /01 input/ESDProtection8/O4 -> /01 input/ESDProtection10/O3
- R80 pad 1: +3V3 -> /01 input/ESDProtection10/O4
- R80 pad 2: SDA1 -> Net-(R76-Pad1)
- R81 pad 1: +3V3 -> Net-(R81-Pad1)
- R81 pad 2: SCL1 -> /01 input/ESDProtection11/I1
- SW4 pad 1: Net-(R24-Pad1) -> Net-(R136-Pad1)
- U1 pad 1: /02 output/PA10 -> /01 input/PC1
- U1 pad 10: (no net) -> /01 input/ESDProtection4/O1
- U1 pad 11: /02 output/O1.1 -> /01 input/ESDProtection3/O2
- U1 pad 12: /02 output/O1.2 -> GND
- U1 pad 13: /02 output/O1.3 -> /01 input/ESDProtection1/O1
- U1 pad 14: /02 output/O1.4 -> /01 input/ESDProtection2/O2
- U1 pad 15: /02 output/O1.5 -> /01 input/ESDProtection2/O3
- U1 pad 16: /02 output/O1.6 -> /01 input/ESDProtection1/O4
- U1 pad 17: /02 output/O1.7 -> /01 input/ESDProtection1/O2
- U1 pad 18: /02 output/O1.8 -> /01 input/ESDProtection2/O1
- U1 pad 2: /02 output/PA9 -> +3V3
- U1 pad 3: /02 output/PA8 -> +3V3
- U1 pad 4: /02 output/PC9 -> /01 input/ESDProtection3/O4
- U1 pad 5: /02 output/PC7 -> /01 input/ESDProtection4/O3
- U1 pad 6: /02 output/PC6 -> /01 input/ESDProtection4/O2
- U1 pad 7: /02 output/PB15 -> /01 input/ESDProtection3/O1
- U1 pad 8: /02 output/PB14 -> /01 input/ESDProtection3/O3
- U1 pad 9: GND -> /01 input/ESDProtection4/O4
- U10 pad 1: Net-(R2-Pad1) -> Net-(R42-Pad1)
- U10 pad 3: Net-(R3-Pad1) -> Net-(R43-Pad1)
- U10 pad 4: Net-(R4-Pad1) -> Net-(R44-Pad1)
- U10 pad 6: Net-(R1-Pad1) -> Net-(R41-Pad1)
- U11 pad 1: Net-(R10-Pad1) -> Net-(R50-Pad1)
- U11 pad 3: Net-(R11-Pad1) -> Net-(R51-Pad1)
- U11 pad 4: Net-(R12-Pad1) -> Net-(R52-Pad1)
- U11 pad 6: Net-(R13-Pad2) -> Net-(R49-Pad1)
- U12 pad 1: Net-(R33-Pad1) -> Net-(R58-Pad1)
- U12 pad 3: Net-(R34-Pad1) -> Net-(R59-Pad1)
- U12 pad 4: Net-(R35-Pad1) -> Net-(R60-Pad1)
- U12 pad 6: Net-(R32-Pad1) -> Net-(R57-Pad1)
- U13 pad 1: Net-(R41-Pad1) -> Net-(R66-Pad1)
- U13 pad 3: Net-(R42-Pad1) -> Net-(R67-Pad1)
- U13 pad 4: Net-(R43-Pad1) -> Net-(R68-Pad1)
- U13 pad 6: Net-(R40-Pad1) -> Net-(R65-Pad1)
- U14 pad 1: Net-(R49-Pad1) -> Net-(R74-Pad1)
- U14 pad 3: Net-(R50-Pad1) -> Net-(R75-Pad1)
- U14 pad 4: Net-(R51-Pad1) -> Net-(R76-Pad1)
- U14 pad 6: Net-(R48-Pad1) -> Net-(R73-Pad1)
- U15 pad 1: Net-(R57-Pad1) -> Net-(R82-Pad1)
- U15 pad 3: Net-(R58-Pad1) -> Net-(R83-Pad1)
- U15 pad 4: Net-(R59-Pad1) -> Net-(R84-Pad1)
- U15 pad 6: Net-(R56-Pad1) -> Net-(R81-Pad1)
- U16 pad 1: Net-(R65-Pad1) -> Net-(R90-Pad1)
- U16 pad 3: Net-(R66-Pad1) -> Net-(R91-Pad1)
- U16 pad 4: Net-(R67-Pad1) -> Net-(R92-Pad1)
- U16 pad 6: Net-(R64-Pad1) -> Net-(R89-Pad1)
- U17 pad 1: Net-(R73-Pad1) -> Net-(R102-Pad2)
- U17 pad 3: Net-(R74-Pad1) -> Net-(R103-Pad2)
- U17 pad 4: Net-(R75-Pad1) -> Net-(R100-Pad1)
- U17 pad 6: Net-(R72-Pad1) -> Net-(R101-Pad2)
- U18 pad 1: /01 input/PC0 -> Net-(R106-Pad1)
- U18 pad 2: +3V3 -> GND
- U18 pad 3: GND -> Net-(R107-Pad1)
- U18 pad 4: /01 input/ESDProtection7/O4 -> Net-(R108-Pad1)
- U18 pad 5: /01 input/ESDProtection8/O3 -> +3V3
- U18 pad 6: /01 input/ESDProtection8/O2 -> Net-(R105-Pad1)
- U19 pad 1: /01 input/PC1 -> Net-(R114-Pad1)
- U19 pad 2: +3V3 -> GND
- U19 pad 3: +3V3 -> Net-(R115-Pad1)
- U19 pad 4: /01 input/ESDProtection3/O4 -> Net-(R116-Pad1)
- U19 pad 5: /01 input/ESDProtection4/O3 -> +3V3
- U19 pad 6: /01 input/ESDProtection4/O2 -> Net-(R113-Pad1)
- U2 pad 1: VCC -> /01 input/PC0
- U2 pad 10: /02 output/O1.15 -> /01 input/ESDProtection8/O1
- U2 pad 11: /02 output/O1.14 -> /01 input/ESDProtection7/O2
- U2 pad 12: /02 output/O1.13 -> GND
- U2 pad 13: /02 output/O1.12 -> /01 input/ESDProtection5/O1
- U2 pad 14: /02 output/O1.11 -> /01 input/ESDProtection6/O2
- U2 pad 15: /02 output/O1.10 -> /01 input/ESDProtection6/O3
- U2 pad 16: /02 output/O1.9 -> /01 input/ESDProtection5/O4
- U2 pad 2: MOSI1 -> GND
- U2 pad 3: SCK1 -> GND
- U2 pad 4: /02 output/PC14 -> /01 input/ESDProtection7/O4
- U2 pad 5: GND -> /01 input/ESDProtection8/O3
- U2 pad 6: Net-(U2-Pad6) -> /01 input/ESDProtection8/O2
- U2 pad 7: (no net) -> /01 input/ESDProtection7/O1
- U2 pad 8: +3V3 -> /01 input/ESDProtection7/O3
- U2 pad 9: /02 output/O1.16 -> /01 input/ESDProtection8/O4
- U20 pad 1: VCC -> Net-(R122-Pad1)
- U20 pad 2: Net-(U20-Pad2) -> GND
- U20 pad 3: SCK1 -> Net-(R123-Pad1)
- U20 pad 4: /02 output/PC14 -> Net-(R124-Pad1)
- U20 pad 5: GND -> +3V3
- U20 pad 6: MISO1 -> Net-(R121-Pad1)
- U3 pad 1: VCC -> /01 input/PC2
- U3 pad 10: /02 output/O1.23 -> /01 input/ESDProtection12/O1
- U3 pad 11: /02 output/O1.22 -> /01 input/ESDProtection11/O2
- U3 pad 12: /02 output/O1.21 -> GND
- U3 pad 13: /02 output/O1.20 -> /01 input/ESDProtection9/O1
- U3 pad 14: /02 output/O1.19 -> /01 input/ESDProtection10/O2
- U3 pad 15: /02 output/O1.18 -> /01 input/ESDProtection10/O3
- U3 pad 16: /02 output/O1.17 -> /01 input/ESDProtection9/O4
- U3 pad 2: Net-(U2-Pad6) -> +3V3
- U3 pad 3: SCK1 -> GND
- U3 pad 4: /02 output/PC14 -> /01 input/ESDProtection11/O4
- U3 pad 5: GND -> /01 input/ESDProtection12/O3
- U3 pad 6: Net-(U20-Pad2) -> /01 input/ESDProtection12/O2
- U3 pad 7: (no net) -> /01 input/ESDProtection11/O1
- U3 pad 8: +3V3 -> /01 input/ESDProtection11/O3
- U3 pad 9: /02 output/O1.24 -> /01 input/ESDProtection12/O4
- U4 pad 1: +3V3 -> /01 input/PC3
- U4 pad 10: /01 input/PC2 -> /01 input/ESDProtection16/O1
- U4 pad 11: /01 input/PC3 -> /01 input/ESDProtection15/O2
- U4 pad 13: Net-(C25-Pad1) -> /01 input/ESDProtection13/O1
- U4 pad 14: /01 input/PA0 -> /01 input/ESDProtection14/O2
- U4 pad 15: /01 input/PA1 -> /01 input/ESDProtection14/O3
- U4 pad 16: /01 input/PA2 -> /01 input/ESDProtection13/O4
- U4 pad 17: /01 input/PA3 -> /01 input/ESDProtection13/O2
- U4 pad 18: GND -> /01 input/ESDProtection14/O1
- U4 pad 19: +3V3 -> /01 input/ESDProtection14/O4
- U4 pad 2: /01 input/PC13 -> +3V3
- U4 pad 20: /01 input/PA4 -> /01 input/ESDProtection13/O3
- U4 pad 21: /01 input/PA5 -> +3V3
- U4 pad 22: /01 input/PA6 -> SCL1
- U4 pad 23: /01 input/PA7 -> SDA1
- U4 pad 24: /01 input/PC4 -> +3V3
- U4 pad 3: /02 output/PC14 -> GND
- U4 pad 4: (no net) -> /01 input/ESDProtection15/O4
- U4 pad 5: Net-(C20-Pad1) -> /01 input/ESDProtection16/O3
- U4 pad 6: Net-(R21-Pad1) -> /01 input/ESDProtection16/O2
- U4 pad 7: /03 cpu/NRST -> /01 input/ESDProtection15/O1
- U4 pad 8: /01 input/PC0 -> /01 input/ESDProtection15/O3
- U4 pad 9: /01 input/PC1 -> /01 input/ESDProtection16/O4
- U5 pad 1: /04 power/V_CB -> Net-(R2-Pad1)
- U5 pad 3: GND -> Net-(R3-Pad1)
- U5 pad 4: +3V3 -> Net-(R4-Pad1)
- U5 pad 5: (no net) -> +3V3
- U5 pad 6: GND -> Net-(R1-Pad1)
- U6 pad 1: CANT -> Net-(R10-Pad1)
- U6 pad 3: +3V3 -> Net-(R11-Pad1)
- U6 pad 4: CANR -> Net-(R12-Pad1)
- U6 pad 5: (no net) -> +3V3
- U6 pad 6: /04 power/CANL -> Net-(R13-Pad2)
- U7 pad 1: GND -> Net-(R18-Pad1)
- U7 pad 3: GND -> Net-(R19-Pad1)
- U7 pad 4: GND -> Net-(R20-Pad1)
- U7 pad 5: GND -> +3V3
- U7 pad 6: Net-(O2-Pad16) -> Net-(R17-Pad1)
- U8 pad 1: +3V3 -> Net-(R26-Pad1)
- U8 pad 2: /03 cpu/1W -> GND
- U8 pad 3: GND -> Net-(R27-Pad1)
- U8 pad 4: SCL2 -> Net-(R28-Pad1)
- U8 pad 5: SDA2 -> +3V3
- U8 pad 6: (no net) -> Net-(R25-Pad1)
- U9 pad 1: +3V3 -> Net-(R34-Pad1)
- U9 pad 2: +3V3 -> GND
- U9 pad 3: +3V3 -> Net-(R35-Pad1)
- U9 pad 4: +3V3 -> Net-(R36-Pad1)
- U9 pad 6: Net-(O2-Pad32) -> Net-(R33-Pad1)
- X1 pad 1: Net-(C20-Pad1) -> Net-(C78-Pad1)
- X1 pad 2: Net-(C21-Pad1) -> Net-(C79-Pad1)
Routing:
- net GND: track 189.2 -> 5.66 mm, vias 33 -> 1
- net +3V3: track 161.4 -> 10.9 mm, vias 13 -> 1
- net VCC: track 134.1 -> 0.00 mm, vias 3 -> 0
- net SDA1: track 107.5 -> 0.00 mm, vias 2 -> 0
- net SCL1: track 107.3 -> 0.00 mm, vias 2 -> 0
- net /03 cpu/DCF77: track 97.6 -> 0.00 mm, vias 2 -> 0
- net /03 cpu/NRST: track 106.2 -> 10.6 mm, vias 2 -> 0
- net /03 cpu/PB2: track 75.5 -> 0.00 mm
- net /03 cpu/PC11: track 63.6 -> 0.00 mm, vias 2 -> 0
- net /01 input/PC0: track 57.3 -> 0.00 mm
- net /03 cpu/PC10: track 56.6 -> 0.00 mm, vias 2 -> 0
- net Net-(R20-Pad1): track 59.2 -> 4.70 mm
- net /02 output/PC14: track 48.9 -> 0.00 mm, vias 5 -> 0
- net SCK1: track 44.5 -> 0.00 mm, vias 1 -> 0
- net /01 input/PC1: track 37.1 -> 0.00 mm, vias 2 -> 0
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- removed copper zone on F.Cu, net /04 power/V_SW
- removed copper zone on B.Cu, net GND
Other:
- board text added: "Antennenmodul intern?"
- board text added: "sensact 2016-09-30 mail@klaus-liebler.de"
- board text removed: "3V3.....GND"
- board text removed: "B6 B7 C13 3V3 GND"
- board text removed: "GND BOOT0 NRST RX"
- board text removed: "sensact 2015-11-07 mail@klaus-liebler.de"
